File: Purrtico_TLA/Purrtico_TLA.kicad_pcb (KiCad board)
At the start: 2 copper layers, 100 x 50 mm, 77 parts, among them J1 XLR3, J3 Conn_01x02, J4 XLR3, J5 Conn_01x02, J7 Conn_02x05_Odd_Even, U1 OPA1679, U2 OPA1679

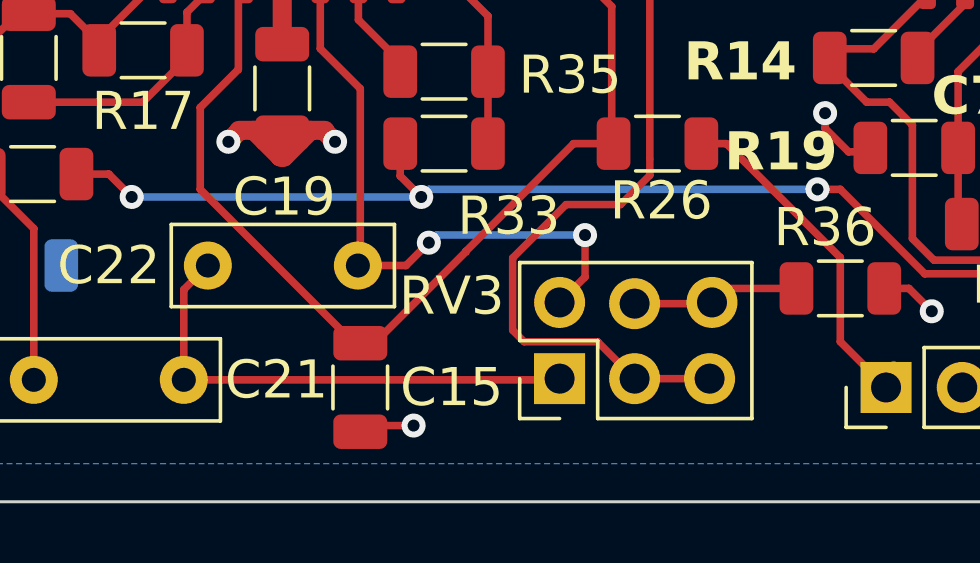
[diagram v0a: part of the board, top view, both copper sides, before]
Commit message: moved rv3
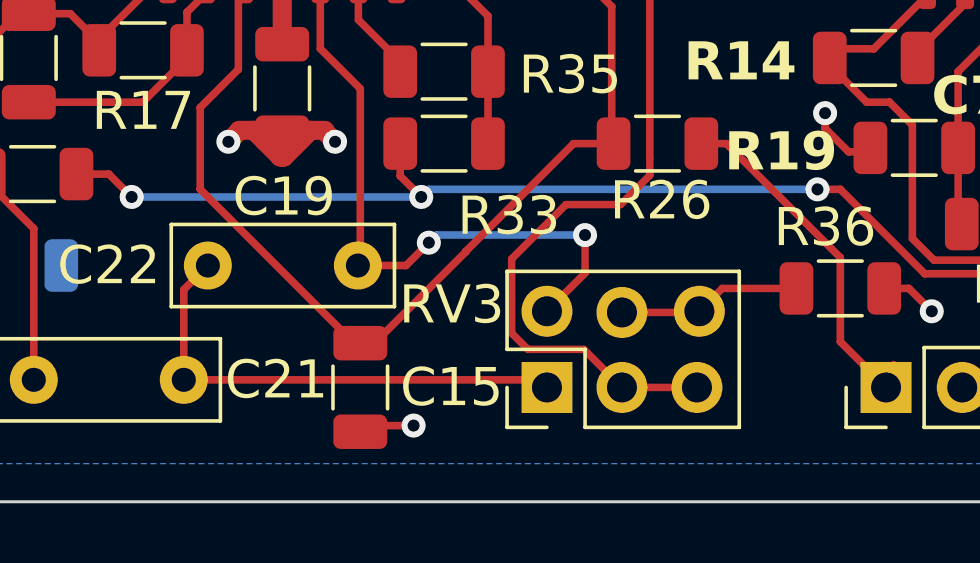
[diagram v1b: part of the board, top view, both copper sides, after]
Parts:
- moved RV3 0.51 mm to (89.5, 78.7)
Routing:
- net Net-(R36-Pad2): track 4.89 -> 6.09 mm
- net Net-(C21-Pad2): track 16.6 -> 16.0 mm
